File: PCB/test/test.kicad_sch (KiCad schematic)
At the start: 52 parts, among them CN1 HEADER_1X10, CN2 HEADER_1X10, CN3 USB_1, CN4 HEADER_1X4, CN5 UFL, SW2 MLL1200S_TE, U1 STM32WBxx_QFN48, U2 USBLC6-2SC6, U3 LD3985M33R, X1 NX2016_32MHz, X2 NX2012_32K768Hz

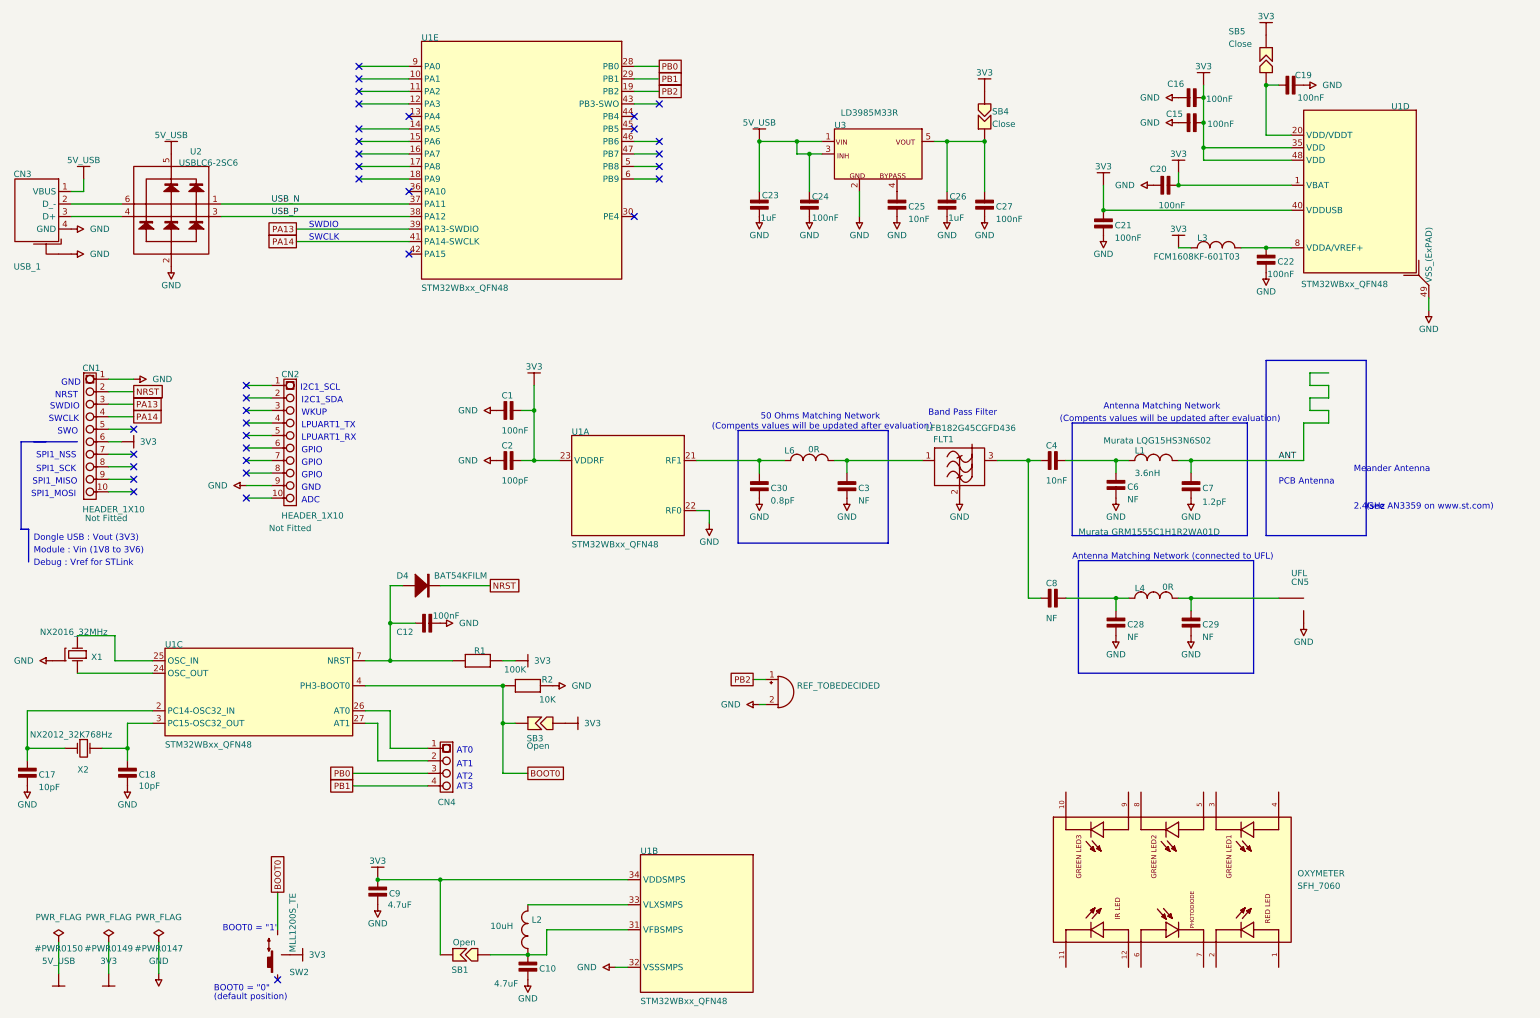
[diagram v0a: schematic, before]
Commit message: schema quasi fini
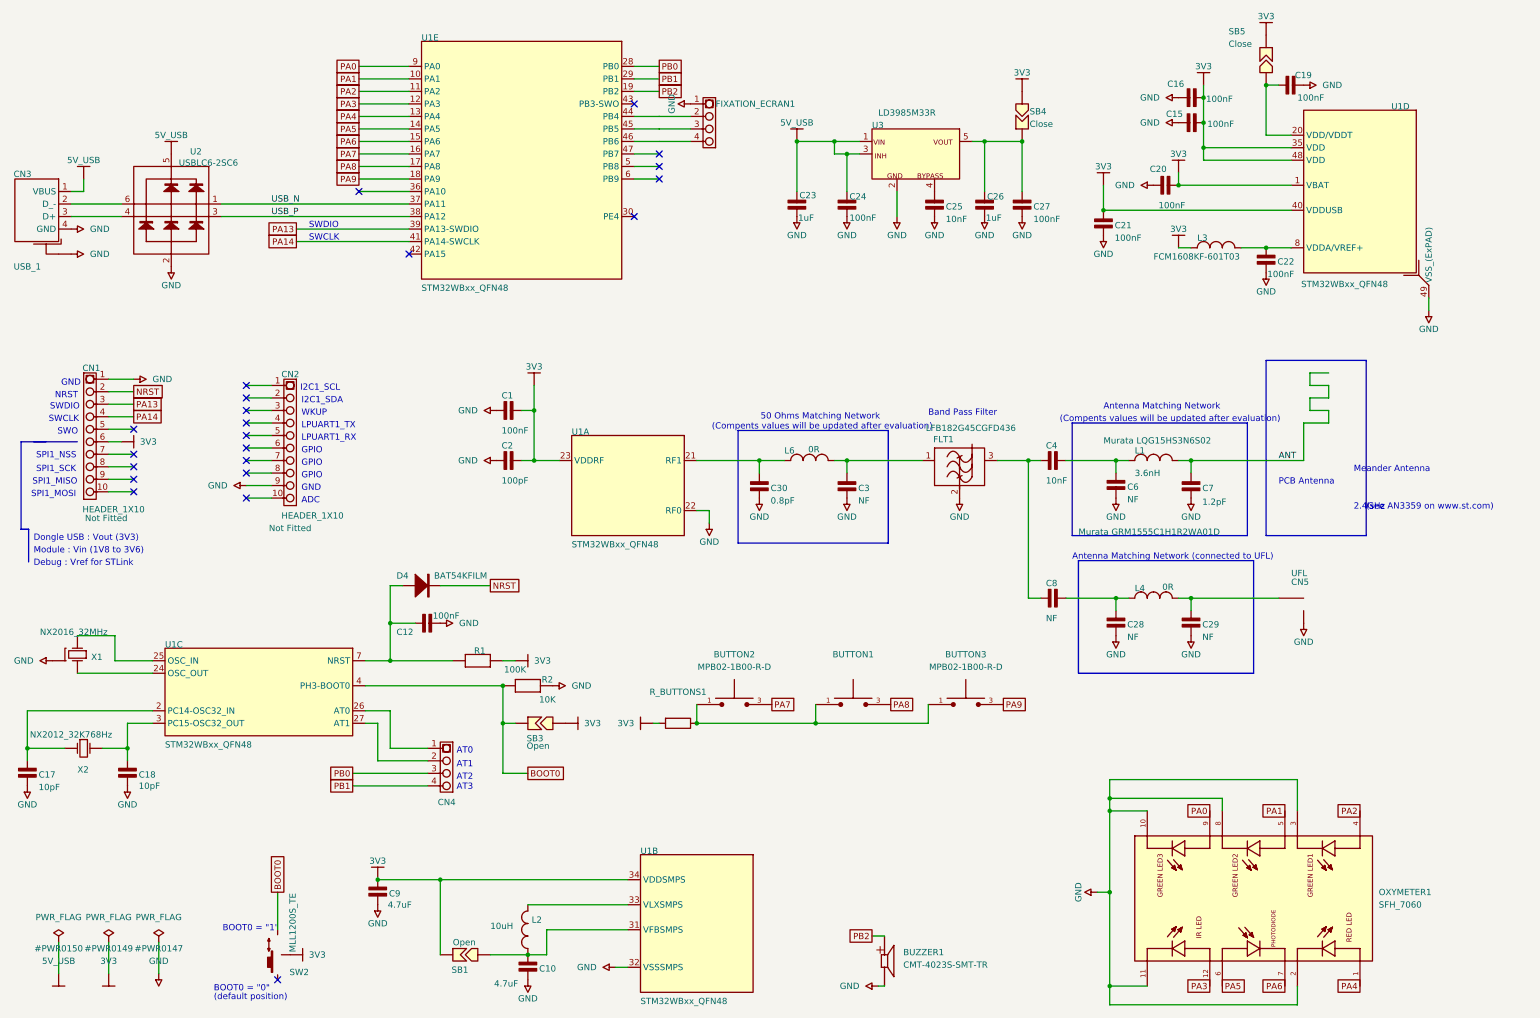
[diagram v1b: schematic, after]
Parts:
- removed REF_TOBEDECIDED: (no value), symbol Device:Buzzer
- added BUTTON1: (no value), symbol MPB02-1B00-R-D:MPB02-1B00-R-D
- added BUTTON2, BUTTON3: MPB02-1B00-R-D, SW_MPB02-1B00-R-D, symbol MPB02-1B00-R-D:MPB02-1B00-R-D
- added BUZZER1: CMT-4023S-SMT-TR, CUI_CMT-4023S-SMT-TR, symbol CMT-4023S-SMT-TR:CMT-4023S-SMT-TR
- added FIXATION_ECRAN1: (no value), symbol test-altium-import:0_mirrored_HEADER_1X4
- added R_BUTTONS1: (no value), symbol Device:R
- renumbered OXYMETER to OXYMETER1
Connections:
- net 3V3: now also R_BUTTONS1.2
- net GND: now also OXYMETER1.10, OXYMETER1.11, OXYMETER1.2, OXYMETER1.3, OXYMETER1.8, BUZZER1.N, FIXATION_ECRAN1.1
- net PB2: now also BUZZER1.P
- net PA1: now reaches U1.10 (PA1)
- net PA1: now also OXYMETER1.5
- net PA2: now reaches U1.11 (PA2)
- net PA2: now also OXYMETER1.4
- net PA3: now reaches U1.12 (PA3)
- net PA3: now also OXYMETER1.12
- net PA4: now reaches U1.13 (PA4)
- net PA4: now also OXYMETER1.1
- net PA5: now reaches U1.14 (PA5)
- net PA5: now also OXYMETER1.6
- net PA6: now reaches U1.15 (PA6)
- net PA6: now also OXYMETER1.7
- net PA7: now reaches U1.16 (PA7)
- net PA7: now also BUTTON2.3
- net PA8: now reaches U1.17 (PA8)
- net PA8: now also BUTTON1.3
- net PA9: now reaches U1.18 (PA9)
- net PA9: now also BUTTON3.3
- net at U1.44 (PB4): now also FIXATION_ECRAN1.2
- net at U1.45 (PB5): now also FIXATION_ECRAN1.3
- net at U1.46 (PB6): now also FIXATION_ECRAN1.4
- net PA0: now reaches U1.9 (PA0)
- net PA0: now also OXYMETER1.9
- new net: BUTTON1.1, BUTTON2.1, BUTTON3.1, R_BUTTONS1.1
- no-connect marks 35 -> 22
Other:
- moved on the sheet: C23, C24, C25, C26, C27, OXYMETER1, SB4, U3
